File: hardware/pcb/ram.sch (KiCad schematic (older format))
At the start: 12 parts, among them U100 XC6SLX16-FTG256, U200 IS66WVE4M16

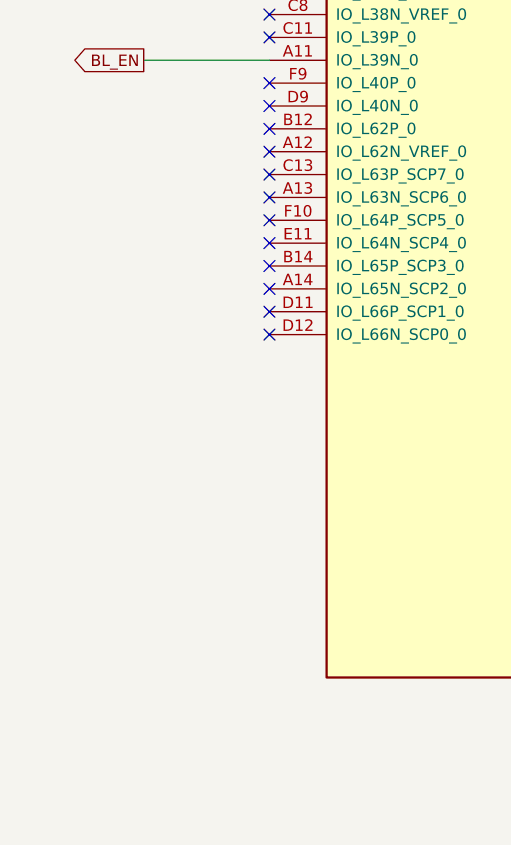
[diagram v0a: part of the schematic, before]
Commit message: vbh: pcb layout
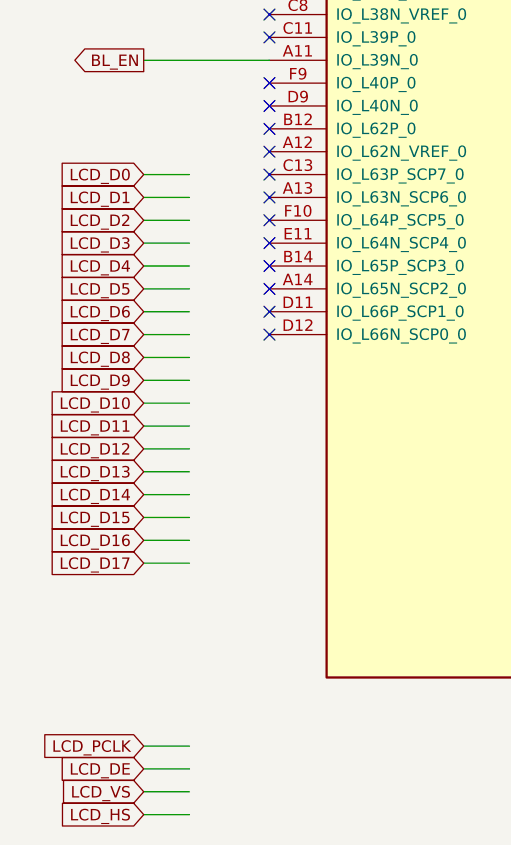
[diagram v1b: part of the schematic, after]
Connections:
- net labels added: LCD_D0, LCD_D1, LCD_D10, LCD_D11, LCD_D12, LCD_D13, LCD_D14, LCD_D15, LCD_D16, LCD_D17, LCD_D2, LCD_D3, LCD_D4, LCD_D5, LCD_D6, LCD_D7, LCD_D8, LCD_D9, LCD_DE, LCD_HS, LCD_PCLK, LCD_VS
- wire segments 147 -> 169
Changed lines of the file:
@@
 NoConn ~ 1700 5500
 NoConn ~ 1700 5600
+Text GLabel 1150 4900 0    50   Input ~ 0
+LCD_D0
+Text GLabel 1150 5000 0    50   Input ~ 0
+LCD_D1
+Text GLabel 1150 5100 0    50   Input ~ 0
+LCD_D2
+Text GLabel 1150 5200 0    50   Input ~ 0
+LCD_D3
+Text GLabel 1150 5300 0    50   Input ~ 0
+LCD_D4
+Text GLabel 1150 5400 0    50   Input ~ 0
+LCD_D5
+Text GLabel 1150 5500 0    50   Input ~ 0
+LCD_D6
+Text GLabel 1150 5600 0    50   Input ~ 0
+LCD_D7
+Text GLabel 1150 5700 0    50   Input ~ 0
+LCD_D8
+Text GLabel 1150 5800 0    50   Input ~ 0
+LCD_D9
+Text GLabel 1150 5900 0    50   Input ~ 0
+LCD_D10
+Text GLabel 1150 6000 0    50   Input ~ 0
+LCD_D11
+Text GLabel 1150 6100 0    50   Input ~ 0
+LCD_D12
+Text GLabel 1150 6200 0    50   Input ~ 0
+LCD_D13
+Text GLabel 1150 6300 0    50   Input ~ 0
+LCD_D14
+Text GLabel 1150 6400 0    50   Input ~ 0
+LCD_D15
+Text GLabel 1150 6500 0    50   Input ~ 0
+LCD_D16
+Text GLabel 1150 6600 0    50   Input ~ 0
+LCD_D17
+Text GLabel 1150 7400 0    50   Input ~ 0
+LCD_PCLK
+Text GLabel 1150 7500 0    50   Input ~ 0
+LCD_DE
+Text GLabel 1150 7600 0    50   Input ~ 0
+LCD_VS
+Text GLabel 1150 7700 0    50   Input ~ 0
+LCD_HS
+Wire Wire Line
+	1150 4900 1350 4900
+Wire Wire Line
+	1150 5000 1350 5000
+Wire Wire Line
+	1150 5100 1350 5100
+Wire Wire Line
+	1150 5200 1350 5200
+Wire Wire Line
+	1150 5300 1350 5300
+Wire Wire Line
+	1150 5400 1350 5400
+Wire Wire Line
+	1150 5500 1350 5500
+Wire Wire Line
+	1150 5600 1350 5600
+Wire Wire Line
+	1150 5700 1350 5700
+Wire Wire Line
+	1150 5800 1350 5800
+Wire Wire Line
+	1150 5900 1350 5900
+Wire Wire Line
+	1150 6000 1350 6000
+Wire Wire Line
+	1150 6100 1350 6100
+Wire Wire Line
+	1150 6200 1350 6200
+Wire Wire Line
+	1150 6300 1350 6300
+Wire Wire Line
+	1150 6400 1350 6400
+Wire Wire Line
+	1150 6500 1350 6500
+Wire Wire Line
+	1150 6600 1350 6600
+Wire Wire Line
+	1150 7400 1350 7400
+Wire Wire Line
+	1150 7500 1350 7500
+Wire Wire Line
+	1150 7600 1350 7600
+Wire Wire Line
+	1150 7700 1350 7700
 $EndSCHEMATC
